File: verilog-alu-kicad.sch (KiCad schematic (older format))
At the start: 9 parts

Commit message: change pin name & add footprint
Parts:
- NAND-IC-1, NAND-IC-2, NAND-IC-3, NAND-IC-4: footprint (none) -> Digikey:Socket_DIP-14_7.62mm_Conn
- gave numbers to parts that had none: 5
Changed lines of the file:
@@
 EESchema Schematic File Version 4
 LIBS:verilog-alu-kicad-cache
-EELAYER 26 0
+EELAYER 30 0
 EELAYER END
 $Descr A4 11693 8268
@@
 F 0 "NAND-IC-1" H 2730 4646 50  0000 L CNN
 F 1 "74LS00" H 2730 4555 50  0000 L CNN
-F 2 "" H 2500 4600 50  0001 C CNN
+F 2 "Digikey:Socket_DIP-14_7.62mm_Conn" H 2500 4600 50  0001 C CNN
 F 3 "http://www.ti.com/lit/gpn/sn74ls00" H 2500 4600 50  0001 C CNN
 	5    2500 4600
@@
 F 0 "NAND-IC-2" H 3580 4646 50  0000 L CNN
 F 1 "74LS00" H 3580 4555 50  0000 L CNN
-F 2 "" H 3350 4600 50  0001 C CNN
+F 2 "Digikey:Socket_DIP-14_7.62mm_Conn" H 3350 4600 50  0001 C CNN
 F 3 "http://www.ti.com/lit/gpn/sn74ls00" H 3350 4600 50  0001 C CNN
 	5    3350 4600
@@
 F 0 "NAND-IC-4" H 9300 3025 50  0000 C CNN
 F 1 "74LS00" H 9300 2934 50  0000 C CNN
-F 2 "" H 9300 2700 50  0001 C CNN
+F 2 "Digikey:Socket_DIP-14_7.62mm_Conn" H 9300 2700 50  0001 C CNN
 F 3 "http://www.ti.com/lit/gpn/sn74ls00" H 9300 2700 50  0001 C CNN
 	4    9300 2700
@@
 F 0 "NAND-IC-4" H 8300 3325 50  0000 C CNN
 F 1 "74LS00" H 8300 3234 50  0000 C CNN
-F 2 "" H 8300 3000 50  0001 C CNN
+F 2 "Digikey:Socket_DIP-14_7.62mm_Conn" H 8300 3000 50  0001 C CNN
 F 3 "http://www.ti.com/lit/gpn/sn74ls00" H 8300 3000 50  0001 C CNN
 	3    8300 3000
@@
 F 0 "NAND-IC-4" H 8300 2775 50  0000 C CNN
 F 1 "74LS00" H 8300 2684 50  0000 C CNN
-F 2 "" H 8300 2450 50  0001 C CNN
+F 2 "Digikey:Socket_DIP-14_7.62mm_Conn" H 8300 2450 50  0001 C CNN
 F 3 "http://www.ti.com/lit/gpn/sn74ls00" H 8300 2450 50  0001 C CNN
 	2    8300 2450
@@
 F 0 "NAND-IC-4" H 7700 4225 50  0000 C CNN
 F 1 "74LS00" H 7700 4134 50  0000 C CNN
-F 2 "" H 7700 3900 50  0001 C CNN
+F 2 "Digikey:Socket_DIP-14_7.62mm_Conn" H 7700 3900 50  0001 C CNN
 F 3 "http://www.ti.com/lit/gpn/sn74ls00" H 7700 3900 50  0001 C CNN
 	1    7700 3900
@@
 F 0 "NAND-IC-2" H 5600 2975 50  0000 C CNN
 F 1 "74LS00" H 5600 2884 50  0000 C CNN
-F 2 "" H 5600 2650 50  0001 C CNN
+F 2 "Digikey:Socket_DIP-14_7.62mm_Conn" H 5600 2650 50  0001 C CNN
 F 3 "http://www.ti.com/lit/gpn/sn74ls00" H 5600 2650 50  0001 C CNN
 	2    5600 2650
@@
 F 0 "NAND-IC-3" H 2650 1425 50  0000 C CNN
 F 1 "74LS00" H 2650 1334 50  0000 C CNN
-F 2 "" H 2650 1100 50  0001 C CNN
+F 2 "Digikey:Socket_DIP-14_7.62mm_Conn" H 2650 1100 50  0001 C CNN
 F 3 "http://www.ti.com/lit/gpn/sn74ls00" H 2650 1100 50  0001 C CNN
 	1    2650 1100
@@
 F 0 "NAND-IC-3" H 6150 2425 50  0000 C CNN
 F 1 "74LS00" H 6150 2334 50  0000 C CNN
-F 2 "" H 6150 2100 50  0001 C CNN
+F 2 "Digikey:Socket_DIP-14_7.62mm_Conn" H 6150 2100 50  0001 C CNN
 F 3 "http://www.ti.com/lit/gpn/sn74ls00" H 6150 2100 50  0001 C CNN
 	3    6150 2100
@@
 F 0 "NAND-IC-2" H 4800 3225 50  0000 C CNN
 F 1 "74LS00" H 4800 3134 50  0000 C CNN
-F 2 "" H 4800 2900 50  0001 C CNN
+F 2 "Digikey:Socket_DIP-14_7.62mm_Conn" H 4800 2900 50  0001 C CNN
 F 3 "http://www.ti.com/lit/gpn/sn74ls00" H 4800 2900 50  0001 C CNN
 	1    4800 2900
@@
 F 0 "NAND-IC-2" H 6700 3225 50  0000 C CNN
 F 1 "74LS00" H 6700 3134 50  0000 C CNN
-F 2 "" H 6700 2900 50  0001 C CNN
+F 2 "Digikey:Socket_DIP-14_7.62mm_Conn" H 6700 2900 50  0001 C CNN
 F 3 "http://www.ti.com/lit/gpn/sn74ls00" H 6700 2900 50  0001 C CNN
 	4    6700 2900
@@
 F 0 "NAND-IC-2" H 5600 3475 50  0000 C CNN
 F 1 "74LS00" H 5600 3384 50  0000 C CNN
-F 2 "" H 5600 3150 50  0001 C CNN
+F 2 "Digikey:Socket_DIP-14_7.62mm_Conn" H 5600 3150 50  0001 C CNN
 F 3 "http://www.ti.com/lit/gpn/sn74ls00" H 5600 3150 50  0001 C CNN
 	3    5600 3150
@@
 F 0 "NAND-IC-1" H 2750 2625 50  0000 C CNN
 F 1 "74LS00" H 2750 2534 50  0000 C CNN
-F 2 "" H 2750 2300 50  0001 C CNN
+F 2 "Digikey:Socket_DIP-14_7.62mm_Conn" H 2750 2300 50  0001 C CNN
 F 3 "http://www.ti.com/lit/gpn/sn74ls00" H 2750 2300 50  0001 C CNN
 	2    2750 2300
@@
 F 0 "NAND-IC-1" H 1800 2875 50  0000 C CNN
 F 1 "74LS00" H 1800 2784 50  0000 C CNN
-F 2 "" H 1800 2550 50  0001 C CNN
+F 2 "Digikey:Socket_DIP-14_7.62mm_Conn" H 1800 2550 50  0001 C CNN
 F 3 "http://www.ti.com/lit/gpn/sn74ls00" H 1800 2550 50  0001 C CNN
 	1    1800 2550
@@
 F 0 "NAND-IC-1" H 2750 3125 50  0000 C CNN
 F 1 "74LS00" H 2750 3034 50  0000 C CNN
-F 2 "" H 2750 2800 50  0001 C CNN
+F 2 "Digikey:Socket_DIP-14_7.62mm_Conn" H 2750 2800 50  0001 C CNN
 F 3 "http://www.ti.com/lit/gpn/sn74ls00" H 2750 2800 50  0001 C CNN
 	3    2750 2800
@@
 F 0 "NAND-IC-1" H 3700 2875 50  0000 C CNN
 F 1 "74LS00" H 3700 2784 50  0000 C CNN
-F 2 "" H 3700 2550 50  0001 C CNN
+F 2 "Digikey:Socket_DIP-14_7.62mm_Conn" H 3700 2550 50  0001 C CNN
 F 3 "http://www.ti.com/lit/gpn/sn74ls00" H 3700 2550 50  0001 C CNN
 	4    3700 2550
@@
 F 0 "NAND-IC-3" H 3700 1525 50  0000 C CNN
 F 1 "74LS00" H 3700 1434 50  0000 C CNN
-F 2 "" H 3700 1200 50  0001 C CNN
+F 2 "Digikey:Socket_DIP-14_7.62mm_Conn" H 3700 1200 50  0001 C CNN
 F 3 "http://www.ti.com/lit/gpn/sn74ls00" H 3700 1200 50  0001 C CNN
 	2    3700 1200
@@
 F 0 "NAND-IC-3" H 4430 4646 50  0000 L CNN
 F 1 "74LS00" H 4430 4555 50  0000 L CNN
-F 2 "" H 4200 4600 50  0001 C CNN
+F 2 "Digikey:Socket_DIP-14_7.62mm_Conn" H 4200 4600 50  0001 C CNN
 F 3 "http://www.ti.com/lit/gpn/sn74ls00" H 4200 4600 50  0001 C CNN
 	5    4200 4600
@@
 F 0 "NAND-IC-4" H 5230 4646 50  0000 L CNN
 F 1 "74LS00" H 5230 4555 50  0000 L CNN
-F 2 "" H 5000 4600 50  0001 C CNN
+F 2 "Digikey:Socket_DIP-14_7.62mm_Conn" H 5000 4600 50  0001 C CNN
 F 3 "http://www.ti.com/lit/gpn/sn74ls00" H 5000 4600 50  0001 C CNN
 	5    5000 4600
@@
 	4200 5100 5000 5100
 $Comp
-L Connector_Generic_MountingPin:Conn_01x02_MountingPin J?
+L Connector_Generic_MountingPin:Conn_01x02_MountingPin decoder_2&decoder_4
 U 1 1 5DEF4F14
 P 1050 2600
-F 0 "J?" H 1138 2423 50  0000 L CNN
+F 0 "decoder_2&decoder_4" H 1138 2423 50  0000 L CNN
 F 1 "Conn_01x02_MountingPin" H 1138 2514 50  0000 L CNN
 F 2 "" H 1050 2600 50  0001 C CNN
@@
 $EndComp
 $Comp
-L Connector_Generic_MountingPin:Conn_01x02_MountingPin J?
+L Connector_Generic_MountingPin:Conn_01x02_MountingPin VCC&GND
 U 1 1 5DEFA690
 P 1650 4500
-F 0 "J?" H 1738 4323 50  0000 L CNN
+F 0 "VCC&GND" H 1738 4323 50  0000 L CNN
 F 1 "Conn_01x02_MountingPin" H 1738 4414 50  0000 L CNN
 F 2 "" H 1650 4500 50  0001 C CNN
@@
 	2350 1150 2350 1200
 $Comp
-L Connector_Generic_MountingPin:Conn_01x02_MountingPin J?
+L Connector_Generic_MountingPin:Conn_01x02_MountingPin InputSelector&OutputSelector
+U 1 1 5DF16C36
+P 1900 1650
+F 0 "InputSelector&OutputSelector" H 1988 1473 50  0000 L CNN
+F 1 "Conn_01x02_MountingPin" H 1988 1564 50  0000 L CNN
+F 2 "" H 1900 1650 50  0001 C CNN
+F 3 "~" H 1900 1650 50  0001 C CNN
+	1    1900 1650
+	-1   0    0    1
+$EndComp
+Wire Wire Line
+	2100 1550 3400 1550
+Wire Wire Line
+	3400 1300 3400 1550
+Wire Wire Line
+	2100 2550 2450 2550
+Connection ~ 7150 3800
+Wire Wire Line
+	2100 1650 2200 1650
+Wire Wire Line
+	2200 3800 7150 3800
+Wire Wire Line
+	2200 1650 2200 3800
+$Comp
+L Connector_Generic_MountingPin:Conn_01x02_MountingPin Cout&Sout
+U 1 1 5DF32BB6
+P 10400 2600
+F 0 "Cout&Sout" H 10487 2516 50  0000 L CNN
+F 1 "Conn_01x02_MountingPin" H 10487 2425 50  0000 L CNN
+F 2 "" H 10400 2600 50  0001 C CNN
+F 3 "~" H 10400 2600 50  0001 C CNN
+	1    10400 2600
+	1    0    0    -1
+$EndComp
+Wire Wire Line
+	7450 2100 10200 2100
+Wire Wire Line
+	10200 2100 10200 2600
+Connection ~ 7450 2100
+Wire Wire Line
+	9600 2700 10200 2700
+$Comp
+L Connector_Generic_MountingPin:Conn_01x02_MountingPin C&decoder_0
 U 1 1 5DF0DD07
 P 1900 1150
-F 0 "J?" H 1988 973 50  0000 L CNN
+F 0 "C&decoder_0" H 1988 973 50  0000 L CNN
 F 1 "Conn_01x02_MountingPin" H 1988 1064 50  0000 L CNN
 F 2 "" H 1900 1150 50  0001 C CNN
@@
 	-1   0    0    1
 $EndComp
-$Comp
-L Connector_Generic_MountingPin:Conn_01x02_MountingPin J?
-U 1 1 5DF16C36
-P 1900 1650
-F 0 "J?" H 1988 1473 50  0000 L CNN
-F 1 "Conn_01x02_MountingPin" H 1988 1564 50  0000 L CNN
-F 2 "" H 1900 1650 50  0001 C CNN
-F 3 "~" H 1900 1650 50  0001 C CNN
-	1    1900 1650
-	-1   0    0    1
-$EndComp
-Wire Wire Line
-	2100 1550 3400 1550
-Wire Wire Line
-	3400 1300 3400 1550
-Wire Wire Line
-	2100 2550 2450 2550
-Connection ~ 7150 3800
-Wire Wire Line
-	2100 1650 2200 1650
-Wire Wire Line
-	2200 3800 7150 3800
-Wire Wire Line
-	2200 1650 2200 3800
-$Comp
-L Connector_Generic_MountingPin:Conn_01x02_MountingPin J?
-U 1 1 5DF32BB6
-P 10400 2600
-F 0 "J?" H 10487 2516 50  0000 L CNN
-F 1 "Conn_01x02_MountingPin" H 10487 2425 50  0000 L CNN
-F 2 "" H 10400 2600 50  0001 C CNN
-F 3 "~" H 10400 2600 50  0001 C CNN
-	1    10400 2600
-	1    0    0    -1
-$EndComp
-Wire Wire Line
-	7450 2100 10200 2100
-Wire Wire Line
-	10200 2100 10200 2600
-Connection ~ 7450 2100
-Wire Wire Line
-	9600 2700 10200 2700
 $EndSCHEMATC

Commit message: add pcb
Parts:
- C&decoder_0, decoder_2&decoder_4: footprint (none) -> Connector_PinHeader_2.54mm:PinHeader_1x03_P2.54mm_Horizontal
- Cout&Sout1: renamed from Cout&Sout; footprint (none) -> Connector_PinHeader_2.54mm:PinHeader_1x03_P2.54mm_Horizontal
- InputSelector&OutputSelector1: renamed from InputSelector&OutputSelector; footprint (none) -> Connector_PinHeader_2.54mm:PinHeader_1x03_P2.54mm_Horizontal
- VCC&GND1: renamed from VCC&GND; footprint (none) -> Connector_PinHeader_2.54mm:PinHeader_1x03_P2.54mm_Horizontal
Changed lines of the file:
@@
 F 0 "decoder_2&decoder_4" H 1138 2423 50  0000 L CNN
 F 1 "Conn_01x02_MountingPin" H 1138 2514 50  0000 L CNN
-F 2 "" H 1050 2600 50  0001 C CNN
+F 2 "Connector_PinHeader_2.54mm:PinHeader_1x03_P2.54mm_Horizontal" H 1050 2600 50  0001 C CNN
 F 3 "~" H 1050 2600 50  0001 C CNN
 	1    1050 2600
@@
 $EndComp
 $Comp
-L Connector_Generic_MountingPin:Conn_01x02_MountingPin VCC&GND
+L Connector_Generic_MountingPin:Conn_01x02_MountingPin VCC&GND1
 U 1 1 5DEFA690
 P 1650 4500
-F 0 "VCC&GND" H 1738 4323 50  0000 L CNN
+F 0 "VCC&GND1" H 1738 4323 50  0000 L CNN
 F 1 "Conn_01x02_MountingPin" H 1738 4414 50  0000 L CNN
-F 2 "" H 1650 4500 50  0001 C CNN
+F 2 "Connector_PinHeader_2.54mm:PinHeader_1x03_P2.54mm_Horizontal" H 1650 4500 50  0001 C CNN
 F 3 "~" H 1650 4500 50  0001 C CNN
 	1    1650 4500
@@
 	2350 1150 2350 1200
 $Comp
-L Connector_Generic_MountingPin:Conn_01x02_MountingPin InputSelector&OutputSelector
+L Connector_Generic_MountingPin:Conn_01x02_MountingPin InputSelector&OutputSelector1
 U 1 1 5DF16C36
 P 1900 1650
-F 0 "InputSelector&OutputSelector" H 1988 1473 50  0000 L CNN
+F 0 "InputSelector&OutputSelector1" H 1988 1473 50  0000 L CNN
 F 1 "Conn_01x02_MountingPin" H 1988 1564 50  0000 L CNN
-F 2 "" H 1900 1650 50  0001 C CNN
+F 2 "Connector_PinHeader_2.54mm:PinHeader_1x03_P2.54mm_Horizontal" H 1900 1650 50  0001 C CNN
 F 3 "~" H 1900 1650 50  0001 C CNN
 	1    1900 1650
@@
 	2200 1650 2200 3800
 $Comp
-L Connector_Generic_MountingPin:Conn_01x02_MountingPin Cout&Sout
+L Connector_Generic_MountingPin:Conn_01x02_MountingPin Cout&Sout1
 U 1 1 5DF32BB6
 P 10400 2600
-F 0 "Cout&Sout" H 10487 2516 50  0000 L CNN
+F 0 "Cout&Sout1" H 10487 2516 50  0000 L CNN
 F 1 "Conn_01x02_MountingPin" H 10487 2425 50  0000 L CNN
-F 2 "" H 10400 2600 50  0001 C CNN
+F 2 "Connector_PinHeader_2.54mm:PinHeader_1x03_P2.54mm_Horizontal" H 10400 2600 50  0001 C CNN
 F 3 "~" H 10400 2600 50  0001 C CNN
 	1    10400 2600
@@
 F 0 "C&decoder_0" H 1988 973 50  0000 L CNN
 F 1 "Conn_01x02_MountingPin" H 1988 1064 50  0000 L CNN
-F 2 "" H 1900 1150 50  0001 C CNN
+F 2 "Connector_PinHeader_2.54mm:PinHeader_1x03_P2.54mm_Horizontal" H 1900 1150 50  0001 C CNN
 F 3 "~" H 1900 1150 50  0001 C CNN
 	1    1900 1150

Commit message: fix pin
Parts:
- removed C&decoder_0, Cout&Sout1, InputSelector&OutputSelector1, VCC&GND1, decoder_2&decoder_4: Conn_01x02_MountingPin, Connector_PinHeader_2.54mm:PinHeader_1x03_P2.54mm_Horizontal, symbol Connector_Generic_MountingPin:Conn_01x02_MountingPin
- added C&decoder_0, Cout&Sout, InputSelector&OutputSelector, JVCC&GND, decoder_2&decoder_4: Conn_01x02, symbol Connector_Generic:Conn_01x02

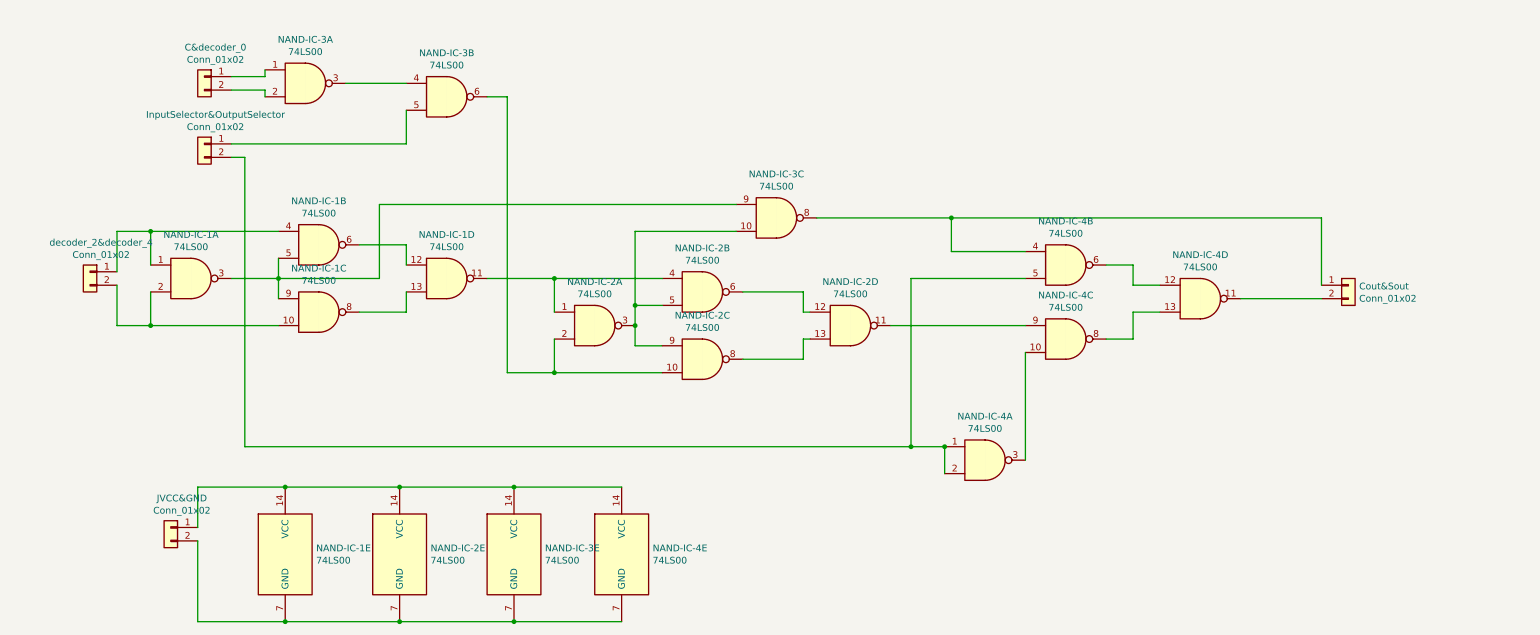
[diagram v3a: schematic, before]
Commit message: try wiring
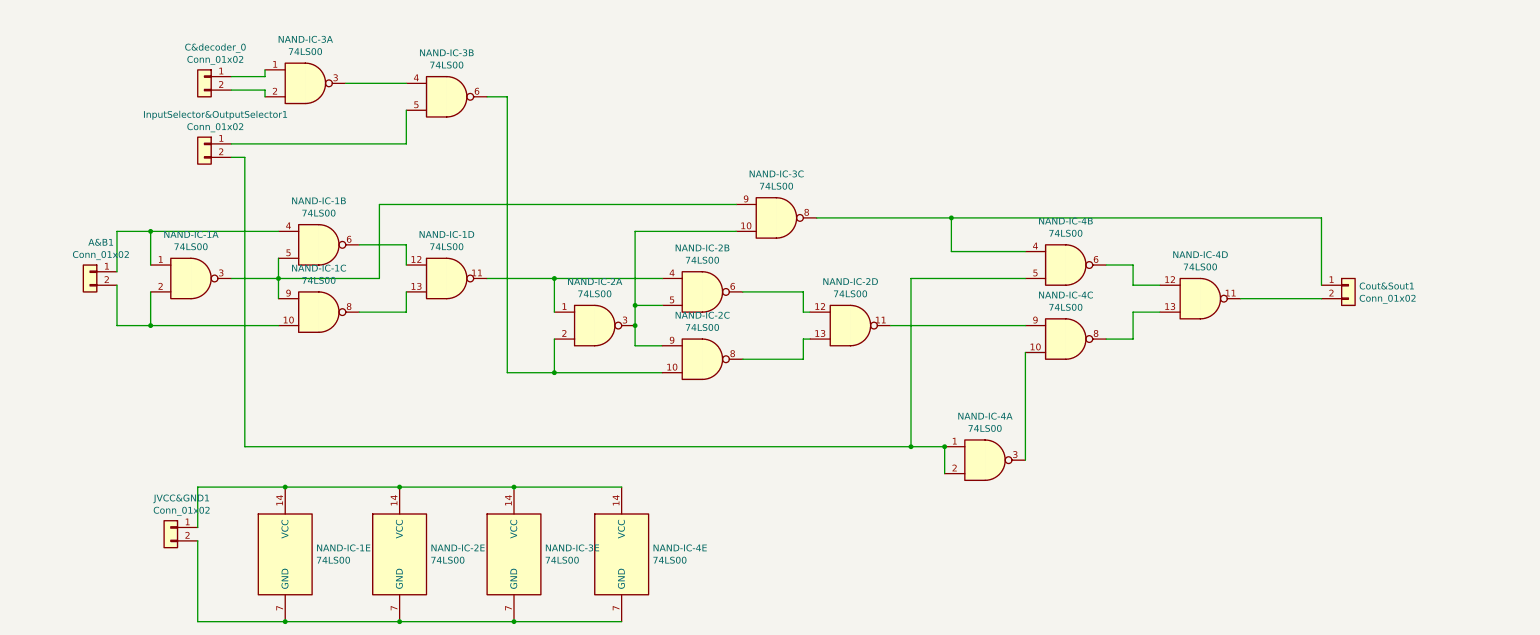
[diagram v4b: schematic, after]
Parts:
- A&B1: renamed from decoder_2&decoder_4; footprint (none) -> Connector_PinHeader_2.54mm:PinHeader_1x02_P2.54mm_Vertical
- C&decoder_0: footprint (none) -> Connector_PinHeader_2.54mm:PinHeader_1x02_P2.54mm_Vertical
- Cout&Sout1: renamed from Cout&Sout; footprint (none) -> Connector_PinHeader_2.54mm:PinHeader_1x02_P2.54mm_Vertical
- InputSelector&OutputSelector1: renamed from InputSelector&OutputSelector; footprint (none) -> Connector_PinHeader_2.54mm:PinHeader_1x02_P2.54mm_Vertical
- JVCC&GND1: renamed from JVCC&GND; footprint (none) -> Connector_PinHeader_2.54mm:PinHeader_1x02_P2.54mm_Vertical
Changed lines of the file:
@@
 $EndComp
 $Comp
-L Connector_Generic:Conn_01x02 JVCC&GND
+L Connector_Generic:Conn_01x02 JVCC&GND1
 U 1 1 5E05D4E7
 P 1650 4400
-F 0 "JVCC&GND" H 1568 4617 50  0000 C CNN
+F 0 "JVCC&GND1" H 1568 4617 50  0000 C CNN
 F 1 "Conn_01x02" H 1568 4526 50  0000 C CNN
-F 2 "" H 1650 4400 50  0001 C CNN
+F 2 "Connector_PinHeader_2.54mm:PinHeader_1x02_P2.54mm_Vertical" H 1650 4400 50  0001 C CNN
 F 3 "~" H 1650 4400 50  0001 C CNN
 	1    1650 4400
@@
 $EndComp
 $Comp
-L Connector_Generic:Conn_01x02 decoder_2&decoder_4
+L Connector_Generic:Conn_01x02 A&B1
 U 1 1 5E0BA8C4
 P 1050 2500
-F 0 "decoder_2&decoder_4" H 968 2717 50  0000 C CNN
+F 0 "A&B1" H 968 2717 50  0000 C CNN
 F 1 "Conn_01x02" H 968 2626 50  0000 C CNN
-F 2 "" H 1050 2500 50  0001 C CNN
+F 2 "Connector_PinHeader_2.54mm:PinHeader_1x02_P2.54mm_Vertical" H 1050 2500 50  0001 C CNN
 F 3 "~" H 1050 2500 50  0001 C CNN
 	1    1050 2500
@@
 $EndComp
 $Comp
-L Connector_Generic:Conn_01x02 InputSelector&OutputSelector
+L Connector_Generic:Conn_01x02 InputSelector&OutputSelector1
 U 1 1 5E0DD4AF
 P 1900 1550
-F 0 "InputSelector&OutputSelector" H 1818 1767 50  0000 C CNN
+F 0 "InputSelector&OutputSelector1" H 1818 1767 50  0000 C CNN
 F 1 "Conn_01x02" H 1818 1676 50  0000 C CNN
-F 2 "" H 1900 1550 50  0001 C CNN
+F 2 "Connector_PinHeader_2.54mm:PinHeader_1x02_P2.54mm_Vertical" H 1900 1550 50  0001 C CNN
 F 3 "~" H 1900 1550 50  0001 C CNN
 	1    1900 1550
@@
 F 0 "C&decoder_0" H 1818 1267 50  0000 C CNN
 F 1 "Conn_01x02" H 1818 1176 50  0000 C CNN
-F 2 "" H 1900 1050 50  0001 C CNN
+F 2 "Connector_PinHeader_2.54mm:PinHeader_1x02_P2.54mm_Vertical" H 1900 1050 50  0001 C CNN
 F 3 "~" H 1900 1050 50  0001 C CNN
 	1    1900 1050
@@
 $EndComp
 $Comp
-L Connector_Generic:Conn_01x02 Cout&Sout
+L Connector_Generic:Conn_01x02 Cout&Sout1
 U 1 1 5E1AD419
 P 10400 2600
-F 0 "Cout&Sout" H 10480 2592 50  0000 L CNN
+F 0 "Cout&Sout1" H 10480 2592 50  0000 L CNN
 F 1 "Conn_01x02" H 10480 2501 50  0000 L CNN
-F 2 "" H 10400 2600 50  0001 C CNN
+F 2 "Connector_PinHeader_2.54mm:PinHeader_1x02_P2.54mm_Vertical" H 10400 2600 50  0001 C CNN
 F 3 "~" H 10400 2600 50  0001 C CNN
 	1    10400 2600
